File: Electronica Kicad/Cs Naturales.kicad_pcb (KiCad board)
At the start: 2 copper layers, 16 parts

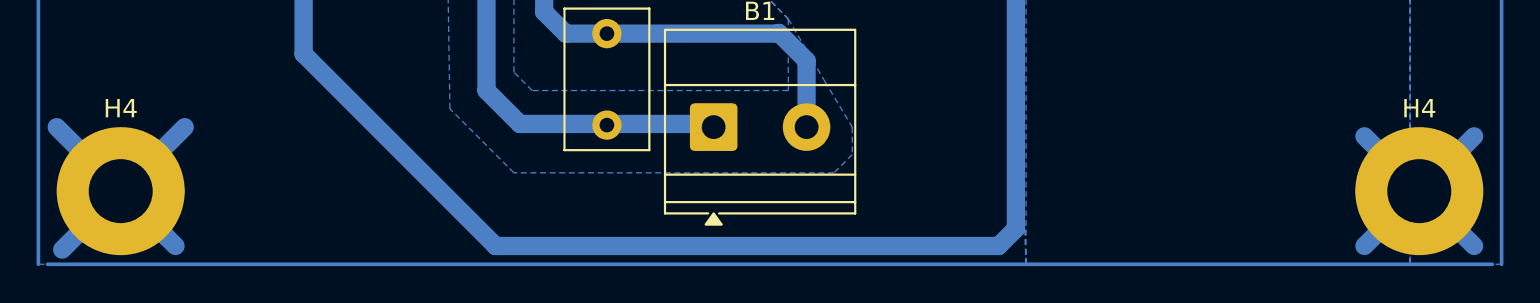
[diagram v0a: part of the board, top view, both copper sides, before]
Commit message: Ordenado
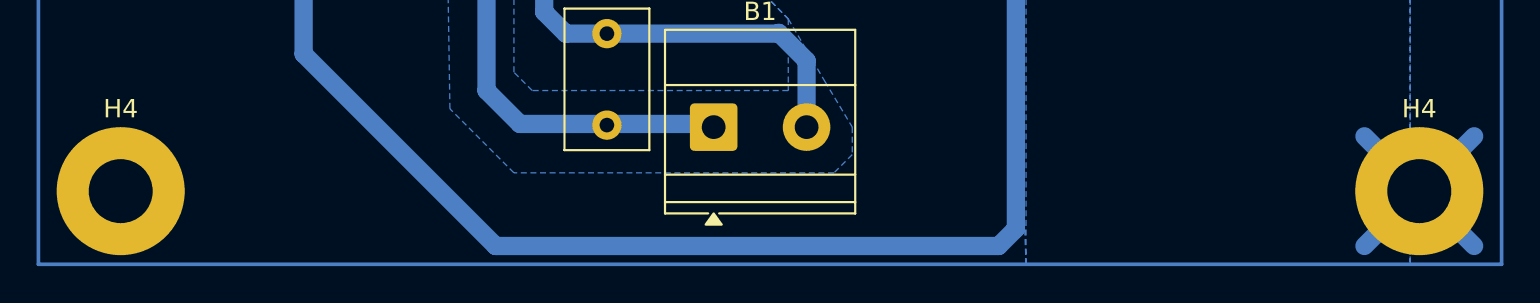
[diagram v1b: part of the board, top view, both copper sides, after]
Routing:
- net GND: track 299.6 -> 201.8 mm
- net S1 +: track 297.8 -> 373.5 mm
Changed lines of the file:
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@@
 	)
 	(gr_line
-		(start 62 138)
-		(end 141 138)
+		(start 61.5 138)
+		(end 141.5 138)
 		(stroke
 			(width 0.2)
@@
 		)
 		(layer "B.Cu")
-		(net 2)
+		(net 7)
 	)
 	(gr_line
@@
 	)
 	(segment
-		(start 65.5 62)
-		(end 62.5 59)
-		(width 1)
-		(layer "B.Cu")
-		(net 2)
-	)
-	(segment
-		(start 61.5 58.5)
-		(end 61.5 138)
-		(width 0.2)
-		(layer "B.Cu")
-		(net 2)
-	)
-	(segment
 		(start 125 96.04)
 		(end 122.54 96.04)
@@
 	)
 	(segment
-		(start 69 65.5)
-		(end 65.5 62)
-		(width 1)
-		(layer "B.Cu")
-		(net 2)
-	)
-	(segment
 		(start 83.5 60)
 		(end 82.5 61)
@@
 		(start 109.1931 110.1931)
 		(end 114.944 110.1931)
-		(width 1)
-		(layer "B.Cu")
-		(net 2)
-	)
-	(segment
-		(start 65.5 62)
-		(end 68.5 59)
 		(width 1)
 		(layer "B.Cu")
@@
 		(start 122.5 96)
 		(end 120.5 98)
-		(width 1)
-		(layer "B.Cu")
-		(net 2)
-	)
-	(segment
-		(start 65.5 62)
-		(end 62 65.5)
 		(width 1)
 		(layer "B.Cu")
@@
 	)
 	(segment
+		(start 65.5 62)
+		(end 62.5 59)
+		(width 1)
+		(layer "B.Cu")
+		(net 7)
+	)
+	(segment
 		(start 114.944 112.7331)
 		(end 118.4831 112.7331)
@@
 	)
 	(segment
+		(start 61.5 58.5)
+		(end 61.5 138)
+		(width 0.2)
+		(layer "B.Cu")
+		(net 7)
+	)
+	(segment
+		(start 69 65.5)
+		(end 65.5 62)
+		(width 1)
+		(layer "B.Cu")
+		(net 7)
+	)
+	(segment
 		(start 137 134)
 		(end 134 137)
@@
 	)
 	(segment
-		(start 66 134)
-		(end 62.5 130.5)
-		(width 1)
-		(layer "B.Cu")
-		(net 7)
-	)
-	(segment
 		(start 114.944 112.7331)
 		(end 114.944 136.056)
@@
 	)
 	(segment
+		(start 65.5 62)
+		(end 68.5 59)
+		(width 1)
+		(layer "B.Cu")
+		(net 7)
+	)
+	(segment
 		(start 76 126.5)
 		(end 76 90)
@@
 	)
 	(segment
-		(start 66 134)
-		(end 68.5 136.5)
-		(width 1)
-		(layer "B.Cu")
-		(net 7)
-	)
-	(segment
 		(start 125 93.5)
 		(end 122.5 93.5)
@@
 	)
 	(segment
-		(start 66 134)
-		(end 69.5 130.5)
+		(start 65.5 62)
+		(end 62 65.5)
 		(width 1)
 		(layer "B.Cu")
@@
 		(start 78 88)
 		(end 79.5 88)
-		(width 1)
-		(layer "B.Cu")
-		(net 7)
-	)
-	(segment
-		(start 66 134)
-		(end 69 137)
 		(width 1)
 		(layer "B.Cu")
@@
 		(width 1)
 		(layer "B.Cu")
-		(net 7)
-	)
-	(segment
-		(start 66 134)
-		(end 62.801 137.199)
-		(width 1)
-		(layer "B.Cu")
